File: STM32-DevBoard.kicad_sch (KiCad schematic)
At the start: 55 parts, among them J1 I2C Bus 1, J2 Serial Debugger, J3 USART1, J4 12402012E212A, J5 PJ-002A, Q1 AO3401A, SW1 SW_SPDT, U1 STM32F103C8T6, U2 TPS563209DDCR, U3 USBLC6-2SC6, Y1 16MHz

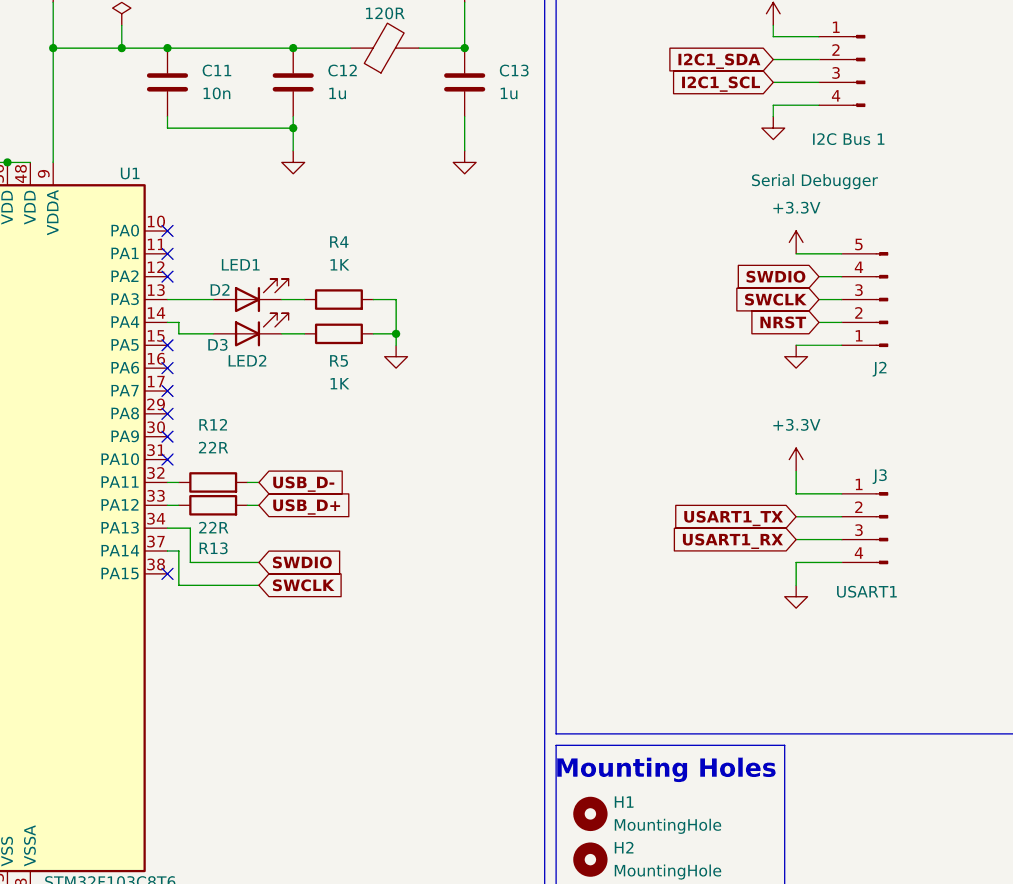
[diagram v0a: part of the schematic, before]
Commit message: extra gpio
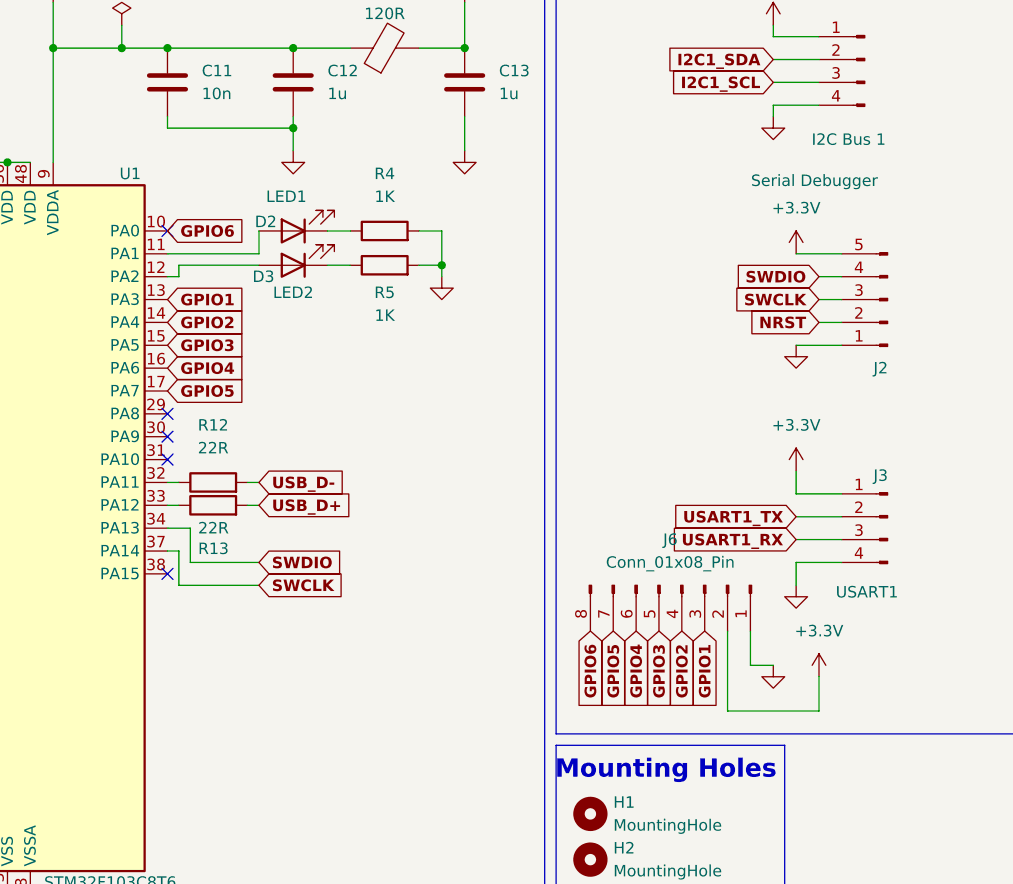
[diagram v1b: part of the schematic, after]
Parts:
- added J6: Conn_01x08_Pin, symbol Connector:Conn_01x08_Pin
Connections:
- net +3.3V: now also J6.2 (Pin_2)
- net GND: now also J6.1 (Pin_1)
- net at D3.2 (A): now also U1.12 (PA2); no longer U1.14 (PA4)
- net GPIO6: now reaches U1.10 (PA0)
- net GPIO6: now also J6.8 (Pin_8)
- net at U1.11 (PA1): now also D2.2 (A)
- net GPIO1: now reaches U1.13 (PA3)
- net GPIO1: now also J6.3 (Pin_3); no longer D2.2 (A)
- net GPIO3: now reaches U1.15 (PA5)
- net GPIO3: now also J6.5 (Pin_5)
- net GPIO4: now reaches U1.16 (PA6)
- net GPIO4: now also J6.6 (Pin_6)
- net GPIO5: now reaches U1.17 (PA7)
- net GPIO5: now also J6.7 (Pin_7)
- new net GPIO2: J6.4 (Pin_4), U1.14 (PA4)
- no-connect marks 27 -> 22
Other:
- moved on the sheet: D2, D3, R4, R5
